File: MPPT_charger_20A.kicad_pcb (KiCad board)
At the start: 2 copper layers, 86 x 73.2 mm, 135 parts, among them J1 SOLAR, J2 LOAD, J3 BAT, J4 UEXT, J5 TEMP, J6 Screw_Terminal_1x02, P1 CONN_01X02, P2 USB_B, P3 USB_OTG, Q1 CSD18540Q5B, Q2 CSD18540Q5B, Q3 CSD18540Q5B, Q4 CSD18540Q5B, SW1 SW_PUSH, T1 MMBT3904, T2 MMBT3904, U1 LM5107, U2 STM32F072CB, U4 MCP16331-CH, U5 AP2210-3.3, U6 LM2665, U7 LM358, U8 TJA1042T/3, Y1 8kHz, Y2 ABS25-32.768KHZ-6-T

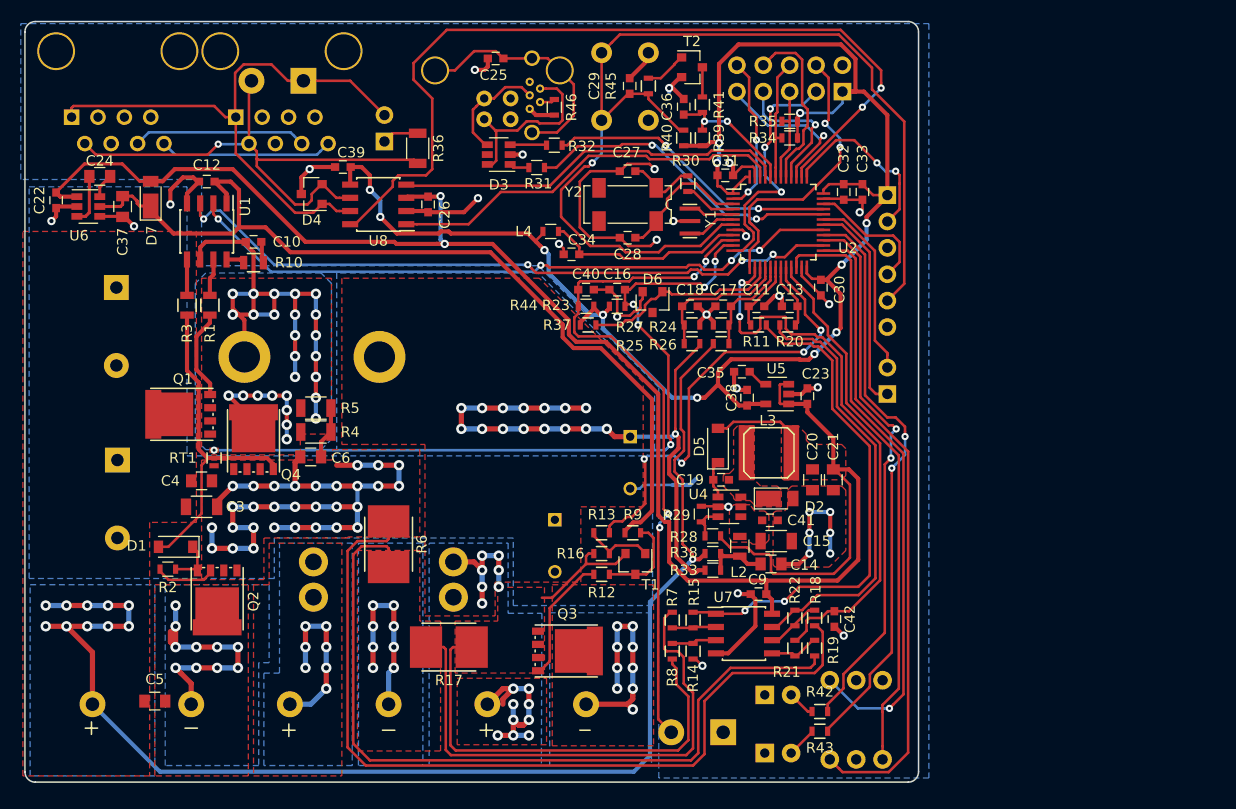
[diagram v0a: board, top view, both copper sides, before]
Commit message: Updated revision: 0.8
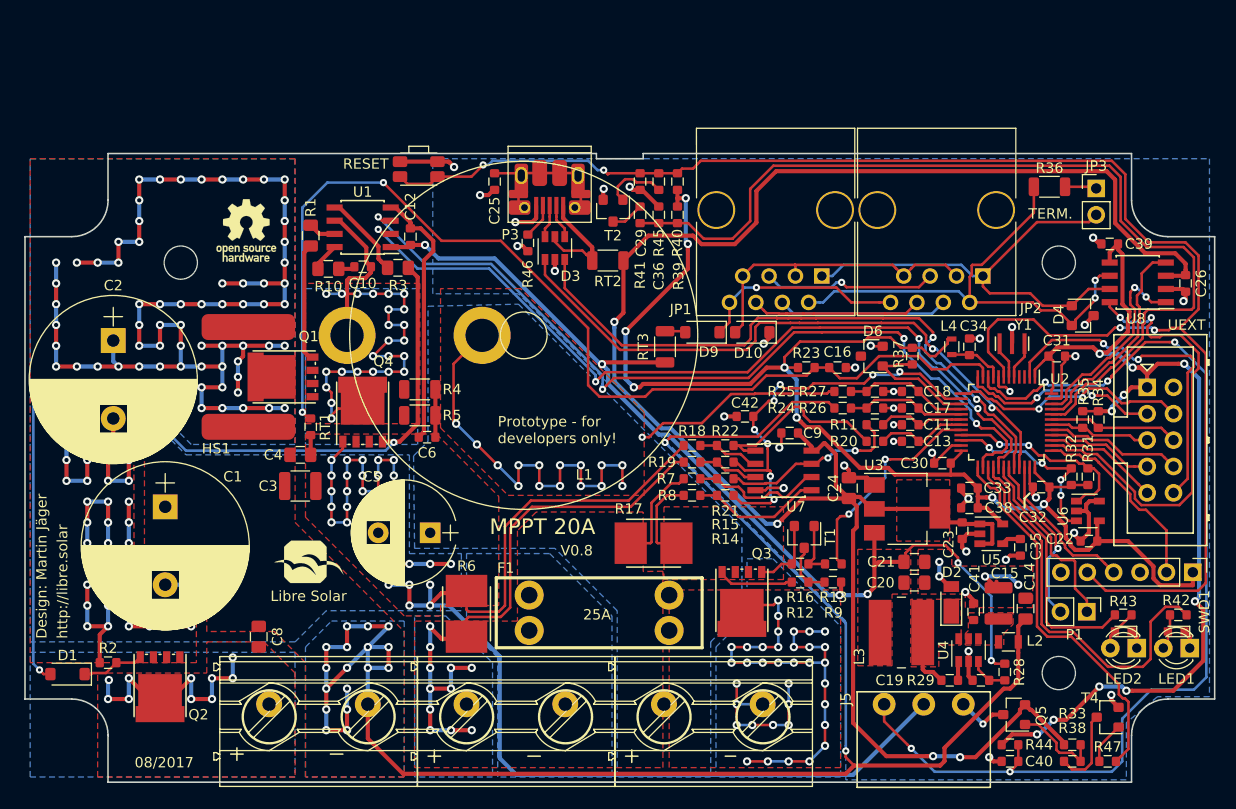
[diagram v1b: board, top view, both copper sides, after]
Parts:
- removed C27, C28: 4.3p, Capacitors_SMD:C_0603
- removed C37: 10u, Capacitors_SMD:C_0805
- removed C7: 820u, Capacitors_THT:C_Radial_D10_L25_P5
- removed D5: 1N4148W-7-F, Diodes_SMD:D_SOD-123
- removed D7: SS16FP, Diodes_SMD:D_PowerDI-123
- removed J6: Screw_Terminal_1x02, Connectors_Terminal_Blocks:TerminalBlock_Pheonix_MKDS1.5-2pol
- removed P2: USB_B, Connectors:USB_B
- removed R30: 0, Resistors_SMD:R_0603
- removed S1: Rotary_Switch, LibreSolar:Rotary_Switch_THT
- removed Y2: ABS25-32.768KHZ-6-T, Crystals:Crystal_SMD_SeikoEpson_MC306-4pin_8.0x3.2mm
- added D10: 1N4148, LibreSolar:D_SOD-123, F.Cu at (168.5, 94.7)
- added D9: 1N4148, LibreSolar:D_SOD-123, F.Cu at (163.7, 94.7)
- added HS1: Heatsink_PAD, LibreSolar:Fischer_Elektronik_FK_250_10_LF_PAK, F.Cu at (120.0, 99.0)
- added LED3: LED, LEDs:LED_0603, F.Cu at (209.3, 123.5)
- added LED4: LED, LEDs:LED_0603, F.Cu at (204.2, 123.5)
- added MK1: Mounting_Hole, Mounting_Holes:MountingHole_3.2mm_M3, F.Cu at (113.5, 88.0)
- added MK2: Mounting_Hole, Mounting_Holes:MountingHole_3.2mm_M3, F.Cu at (198.0, 88.0)
- added MK3: Mounting_Hole, Mounting_Holes:MountingHole_3.2mm_M3, F.Cu at (198.0, 127.5)
- added Q5: BSS84, LibreSolar:SOT-23, F.Cu at (193.7, 131.5)
- added R47: 100k, LibreSolar:R_0603_1608, F.Cu at (202.7, 136.0)
- added RT2: 200mA, LibreSolar:R_1206_3216, F.Cu at (154.6, 87.8)
- added RT3: 200mA, LibreSolar:R_1206_3216, F.Cu at (160.1, 96.1)
- added T4: MMBT3904, LibreSolar:SOT-23, F.Cu at (202.7, 131.8)
- added U3: AZ1117, TO_SOT_Packages_SMD:SOT-223-3Lead_TabPin2, F.Cu at (183.4, 111.7)
- C1, C2, F1, JP3, L1, LED1, LED2, LOGO1, LOGO2, P1, SWD1: moved to F.Cu
- C10, C11, C12, C13, C16, C17, C18, C19, C23, C25, C26, C29, C30, C31, C32, C33, C34, C35, C36, C38, C39, C40, C41, C42, C9: footprint Capacitors_SMD:C_0603 -> LibreSolar:C_0603_1608
- C14, C20, C21, C24, C4: footprint Capacitors_SMD:C_0805 -> LibreSolar:C_0805_2012
- C15: value 4.7u -> 2.2u; footprint Capacitors_SMD:C_1206 -> LibreSolar:C_1210_3225
- C22: value 1u -> 100n; footprint Capacitors_SMD:C_0603 -> LibreSolar:C_0603_1608
- C3: footprint Capacitors_SMD:C_1206 -> LibreSolar:C_1210_3225
- C5: value 1u -> 820u; footprint Capacitors_SMD:C_0805 -> Capacitors_THT:CP_Radial_D10.0mm_P5.00mm
- C6: footprint Capacitors_SMD:C_0805 -> LibreSolar:C_0603_1608
- C8: value 820u -> 1u; footprint Capacitors_THT:C_Radial_D10_L25_P5 -> LibreSolar:C_0805_2012; moved to F.Cu
- D1: value 1N4148W-7-F -> 1N4148; footprint Diodes_SMD:D_SOD-123 -> LibreSolar:D_SOD-123
- D3: footprint TO_SOT_Packages_SMD:SOT-23-6 -> LibreSolar:SOT-23-6
- D4, D6, T1, T2: footprint TO_SOT_Packages_SMD:SOT-23 -> LibreSolar:SOT-23
- J1, J2, J3: footprint LibreSolar:MKDS_5-2-952 -> LibreSolar:Phoenix_Contact_MKDS_5-2-952; moved to F.Cu
- J4: footprint Pin_Headers:Pin_Header_Straight_2x05_Pitch2.54mm -> LibreSolar:Box_Header_2x05x2.54mm_Straight; moved to F.Cu
- J5: value TEMP -> CONN_01X03; footprint Connectors_Terminal_Blocks:TerminalBlock_Pheonix_MKDS1.5-2pol -> LibreSolar:Phoenix_Contact_MC_1,5_3-G-3,81; moved to F.Cu
- JP1, JP2: footprint Connectors:RJ45_8 -> LibreSolar:RJ45_8P8C; moved to F.Cu
- L3: value 22uH -> 47uH; footprint Inductors:SELF-WE-TPC_M -> LibreSolar:L_Wuerth_WE-TPC-58xx
- L4: value L -> 600R
- P3: footprint LibreSolar:Wuerth_USB_Micro_USB_vert_Type_B_614105150721 -> LibreSolar:USB_Micro-B_10103594-0001LF; moved to F.Cu
- R1, R10, R3: footprint Resistors_SMD:R_0805 -> LibreSolar:R_0805_2012
- R11, R12, R13, R14, R15, R16, R18, R19, R2, R20, R21, R22, R23, R24, R25, R26, R27, R29, R34, R35, R37, R39, R40, R41, R42, R43, R44, R45, R46, R7, R8, RT1: footprint Resistors_SMD:R_0603 -> LibreSolar:R_0603_1608
- R28: value 52.3k -> 120k; footprint Resistors_SMD:R_0603 -> LibreSolar:R_0603_1608
- R31, R32: value 0 -> 2.2k; footprint Resistors_SMD:R_0603 -> LibreSolar:R_0603_1608
- R33: value 0 -> 100k; footprint Resistors_SMD:R_0603 -> LibreSolar:R_0603_1608
- R36, R4, R5: footprint Resistors_SMD:R_1206 -> LibreSolar:R_1206_3216
- R38: value 0 -> 1k; footprint Resistors_SMD:R_0603 -> LibreSolar:R_0603_1608
- R9: value 33k -> 56k; footprint Resistors_SMD:R_0603 -> LibreSolar:R_0603_1608
- SW1: footprint Buttons_Switches_THT:SW_PUSH_6mm -> LibreSolar:SW_SPST_EVQP7A; moved to F.Cu
- U4: value MCP16331-CH -> LMR16006X; footprint TO_SOT_Packages_SMD:SOT-23-6 -> LibreSolar:SOT-23-6
- U5: footprint TO_SOT_Packages_SMD:SOT-23-5 -> LibreSolar:SOT-23-5
- U6: value LM2665 -> 24AA01; footprint TO_SOT_Packages_SMD:SOT-23-6 -> TO_SOT_Packages_SMD:SOT-23-5
- moved C22 104.7 mm to (200.9, 114.8), turned to 180 degrees
- moved U6 100.6 mm to (200.8, 111.9)
- moved C24 78.1 mm to (177.8, 109.7), turned to 90 degrees
- moved D4 75.1 mm to (200.3, 93.1), turned to 0 degrees
- moved C39 74.2 mm to (202.9, 86.2)
- moved U8 73.5 mm to (205.6, 89.9)
- moved C26 73.3 mm to (210.2, 90.0)
- moved JP1 68.9 mm to (170.8, 86.8), turned to 180 degrees
- moved JP2 68.7 mm to (186.2, 86.8), turned to 180 degrees
- moved JP3 68.6 mm to (201.6, 80.9)
- moved C40 61.0 mm to (193.3, 136.0), turned to 180 degrees
- moved R36 60.9 mm to (197.1, 80.7), turned to 180 degrees
- moved R31 60.8 mm to (200.8, 108.6), turned to 270 degrees
- moved LOGO1 60.3 mm to (123.5, 118.8), turned to 0 degrees
- moved R32 59.1 mm to (199.2, 108.6), turned to 270 degrees
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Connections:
- net /DCDC power stage/I_DCDC renamed /MCU/I_DCDC
- net /DCDC power stage/I_LOAD renamed /MCU/I_LOAD
- net /DCDC power stage/LOAD-GND renamed /DCDC power stage/LOAD-SW
- net /DCDC power stage/TEMP_INT renamed /Analog Frontend/TEMP_INT
- net /DCDC power stage/V_BAT renamed /MCU/V_BAT
- net /DCDC power stage/V_SOLAR renamed /MCU/V_SOLAR
- C14 pad 1: Net-(C14-Pad1) -> /DCDC power stage/DCDC_IN
- C20 pad 1: +5V -> +10V
- C21 pad 1: +5V -> +10V
- C22 pad 1: +5V -> +3V3
- C24 pad 1: Net-(C24-Pad1) -> +5V
- C24 pad 2: Net-(C24-Pad2) -> GND
- C25 pad 1: /Communication Interfaces/USB_SH -> GND
- C25 pad 2: GND -> Net-(C25-Pad2)
- C40 pad 1: /DCDC power stage/TEMP_BAT -> /Analog Frontend/TEMP_BAT
- C42 pad 1: /DCDC power stage/REF_I_DCDC -> /MCU/DAC
- C5 pad 1: /DCDC power stage/DCDC_IN -> /DCDC power stage/DCDC_OUT
- C5 pad 2: /DCDC power stage/SOLAR- -> GND
- C8 pad 1: /DCDC power stage/DCDC_OUT -> /DCDC power stage/DCDC_IN
- C8 pad 2: GND -> /DCDC power stage/SOLAR-
- D3 pad 1: Net-(D3-Pad1) -> /Communication Interfaces/USB_DP
- D3 pad 3: Net-(D3-Pad3) -> /Communication Interfaces/USB_DM
- D3 pad 5: (no net) -> Net-(D3-Pad5)
- J2 pad 1: /DCDC power stage/LOAD- -> /DCDC power stage/DCDC_OUT
- J2 pad 2: /DCDC power stage/DCDC_OUT -> /DCDC power stage/LOAD-
- J5 pad 1: GND -> /Analog Frontend/TEMP_BAT
- J5 pad 2: /DCDC power stage/TEMP_BAT -> GND
- JP1 pad 4: (no net) -> /Communication Interfaces/RJ45_4
- JP1 pad 5: (no net) -> /Communication Interfaces/RJ45_5
- JP2 pad 4: (no net) -> /Communication Interfaces/RJ45_4
- JP2 pad 5: (no net) -> /Communication Interfaces/RJ45_5
- L2 pad 1: Net-(C14-Pad1) -> /DCDC power stage/DCDC_IN
- L3 pad 2: +5V -> +10V
- P3 pad 1: (no net) -> Net-(D3-Pad5)
- P3 pad 2: Net-(D3-Pad6) -> Net-(D3-Pad4)
- P3 pad 3: Net-(D3-Pad4) -> Net-(D3-Pad6)
- P3 pad 6: /Communication Interfaces/USB_SH -> Net-(C25-Pad2)
- R14 pad 1: GND -> /MCU/DAC
- R21 pad 2: /DCDC power stage/REF_I_DCDC -> /MCU/DAC
- R28 pad 1: +5V -> +10V
- R31 pad 1: Net-(D3-Pad1) -> /MCU/I2C2_SCL
- R31 pad 2: /Communication Interfaces/USB_DM -> +3V3
- R32 pad 1: Net-(D3-Pad3) -> /MCU/I2C2_SDA
- R32 pad 2: /Communication Interfaces/USB_DP -> +3V3
- R33 pad 1: Net-(C14-Pad1) -> +5V
- R33 pad 2: /DCDC power stage/DCDC_OUT -> Net-(Q5-Pad1)
- R38 pad 1: Net-(C14-Pad1) -> Net-(Q5-Pad1)
- R38 pad 2: /DCDC power stage/DCDC_IN -> Net-(R38-Pad2)
- R44 pad 2: /DCDC power stage/TEMP_BAT -> /Analog Frontend/TEMP_BAT
- SWD1 pad 6: (no net) -> Net-(SWD1-Pad6)
- U2 pad 10: /DCDC power stage/TEMP_BAT -> /Analog Frontend/TEMP_BAT
- U2 pad 14: /DCDC power stage/REF_I_DCDC -> /MCU/DAC
- U2 pad 21: /MCU/ROT_0 -> /MCU/I2C2_SCL
- U2 pad 22: /MCU/ROT_1 -> /MCU/I2C2_SDA
- U2 pad 25: /MCU/ROT_2 -> /Communication Interfaces/5V_OUT_EN
- U6 pad 1: +5V -> /MCU/I2C2_SCL
- U6 pad 3: Net-(C24-Pad2) -> /MCU/I2C2_SDA
- U6 pad 4: GND -> +3V3
- U6 pad 5: +10V -> GND
- U7 pad 1: Net-(R11-Pad1) -> Net-(R20-Pad1)
- U7 pad 2: Net-(R15-Pad1) -> Net-(R18-Pad1)
- U7 pad 3: Net-(R14-Pad2) -> Net-(R19-Pad1)
- U7 pad 5: Net-(R19-Pad1) -> Net-(R14-Pad2)
- U7 pad 6: Net-(R18-Pad1) -> Net-(R15-Pad1)
- U7 pad 7: Net-(R20-Pad1) -> Net-(R11-Pad1)
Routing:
- net /DCDC power stage/DCDC_IN: track 128.8 -> 315.0 mm, vias 11 -> 88
- net /Analog Frontend/TEMP_BAT: track 0.00 -> 99.2 mm, vias 0 -> 5
- net /DCDC power stage/BAT-: track 145.5 -> 67.9 mm, vias 8 -> 11
- net /MCU/BOOT0: track 13.0 -> 89.4 mm, vias 2 -> 0
- net /DCDC power stage/TEMP_BAT: track 67.2 -> 0.00 mm, vias 4 -> 0
- net +3V3: track 163.0 -> 228.9 mm, vias 12 -> 18
- net GND: track 291.0 -> 355.2 mm, vias 61 -> 108
- net /MCU/ROT_2: track 61.9 -> 0.00 mm
- net /MCU/ROT_1: track 59.1 -> 0.00 mm, vias 1 -> 0
- net /MCU/~RESET: track 99.8 -> 157.6 mm, vias 1 -> 4
- net /DCDC power stage/REF_I_DCDC: track 54.7 -> 0.00 mm, vias 2 -> 0
- net Net-(D1-Pad2): track 32.8 -> 86.0 mm, vias 0 -> 2
- net /MCU/ROT_0: track 52.3 -> 0.00 mm
- net /DCDC power stage/LOAD-: track 19.9 -> 63.8 mm, vias 9 -> 36
- net /MCU/DAC: track 0.00 -> 40.8 mm, vias 0 -> 8
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- added copper zone on F.Cu, net +10V
- removed copper zone on F.Cu, net /DCDC power stage/BAT+
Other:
- board size 86 x 73.2 mm -> 114.5 x 60.5 mm
- rule pad_to_mask_clearance: 0.2 -> 0
- board text added: "08/2017"
- board text added: "3V3"
- board text added: "5V"
- board text added: "GND"
- board text added: "MPPT 20A"
- board text added: "NTC"
- board text added: "RST"
- board text added: "SWCLK"
- board text added: "SWDIO"
- board text added: "V0.8"
- board text removed: "10k NTC"
- board text removed: "H"
- board text removed: "Housing walls"
- board text removed: "L"
- board text removed: "Libre Solar MPPT 20A"
- board text removed: "Made in Fabulous St. Pauli"
- board text removed: "Mode"
- board text removed: "PCB layout for Phoenix Contact DIN rail housing: - Tray: EH 90 F-B/ABS BK9005 - Cover: EH 90 F-C SS/ABS BK9005"
- board text removed: "Temp"
- board text removed: "USB"
- board text removed: "V0.7 (03/2017)"
